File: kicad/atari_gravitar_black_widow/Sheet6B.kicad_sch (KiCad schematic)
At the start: 20 parts

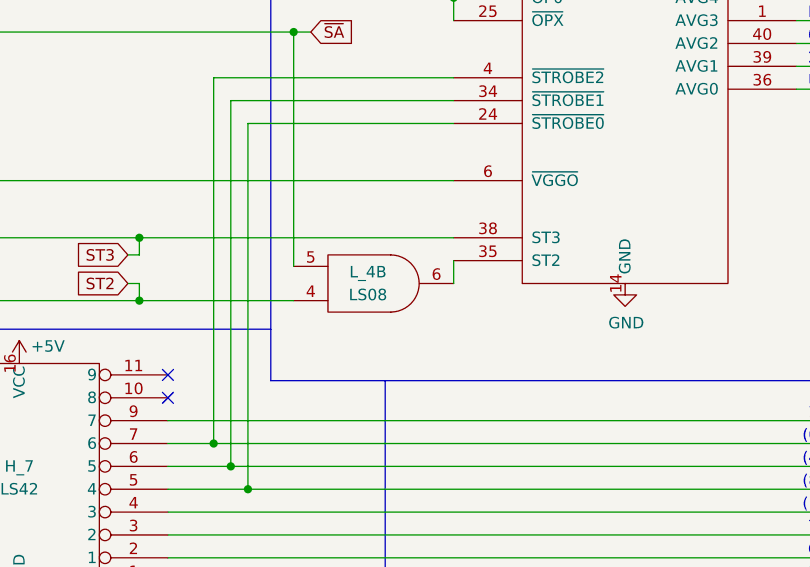
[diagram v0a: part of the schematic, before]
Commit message: 4A DONE
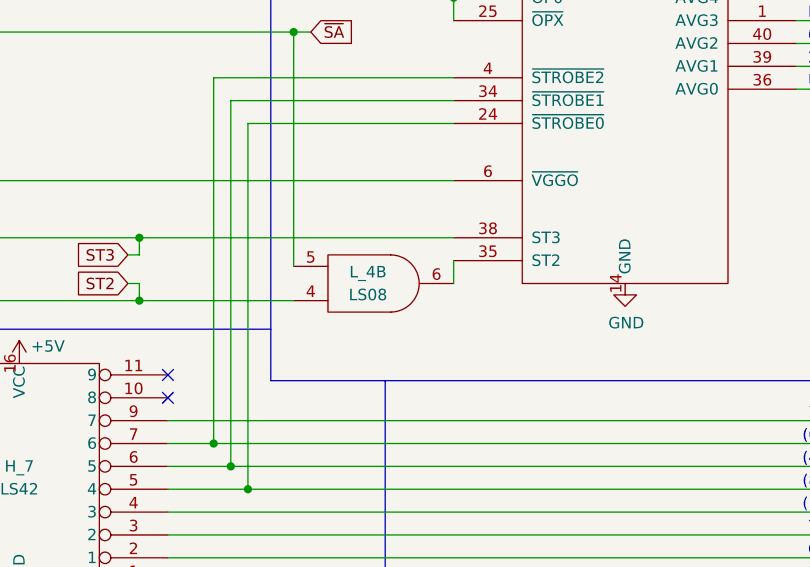
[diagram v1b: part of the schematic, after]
